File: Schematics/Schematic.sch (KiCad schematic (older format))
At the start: 14 parts

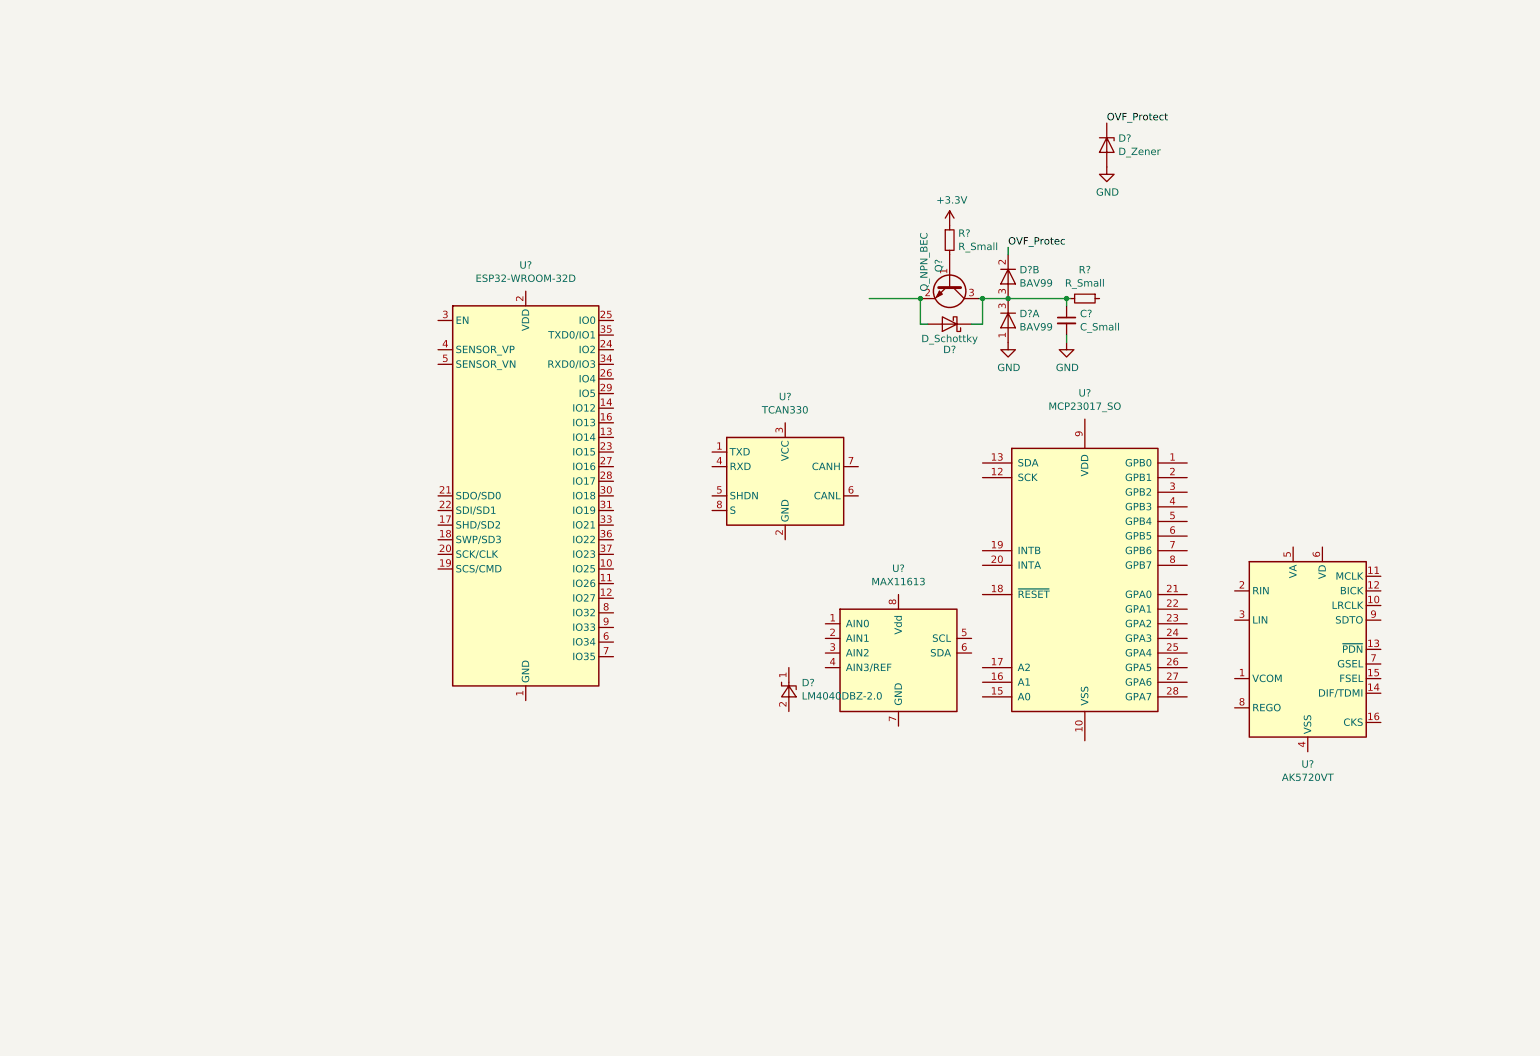
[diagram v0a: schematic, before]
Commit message: Whheee, parts!
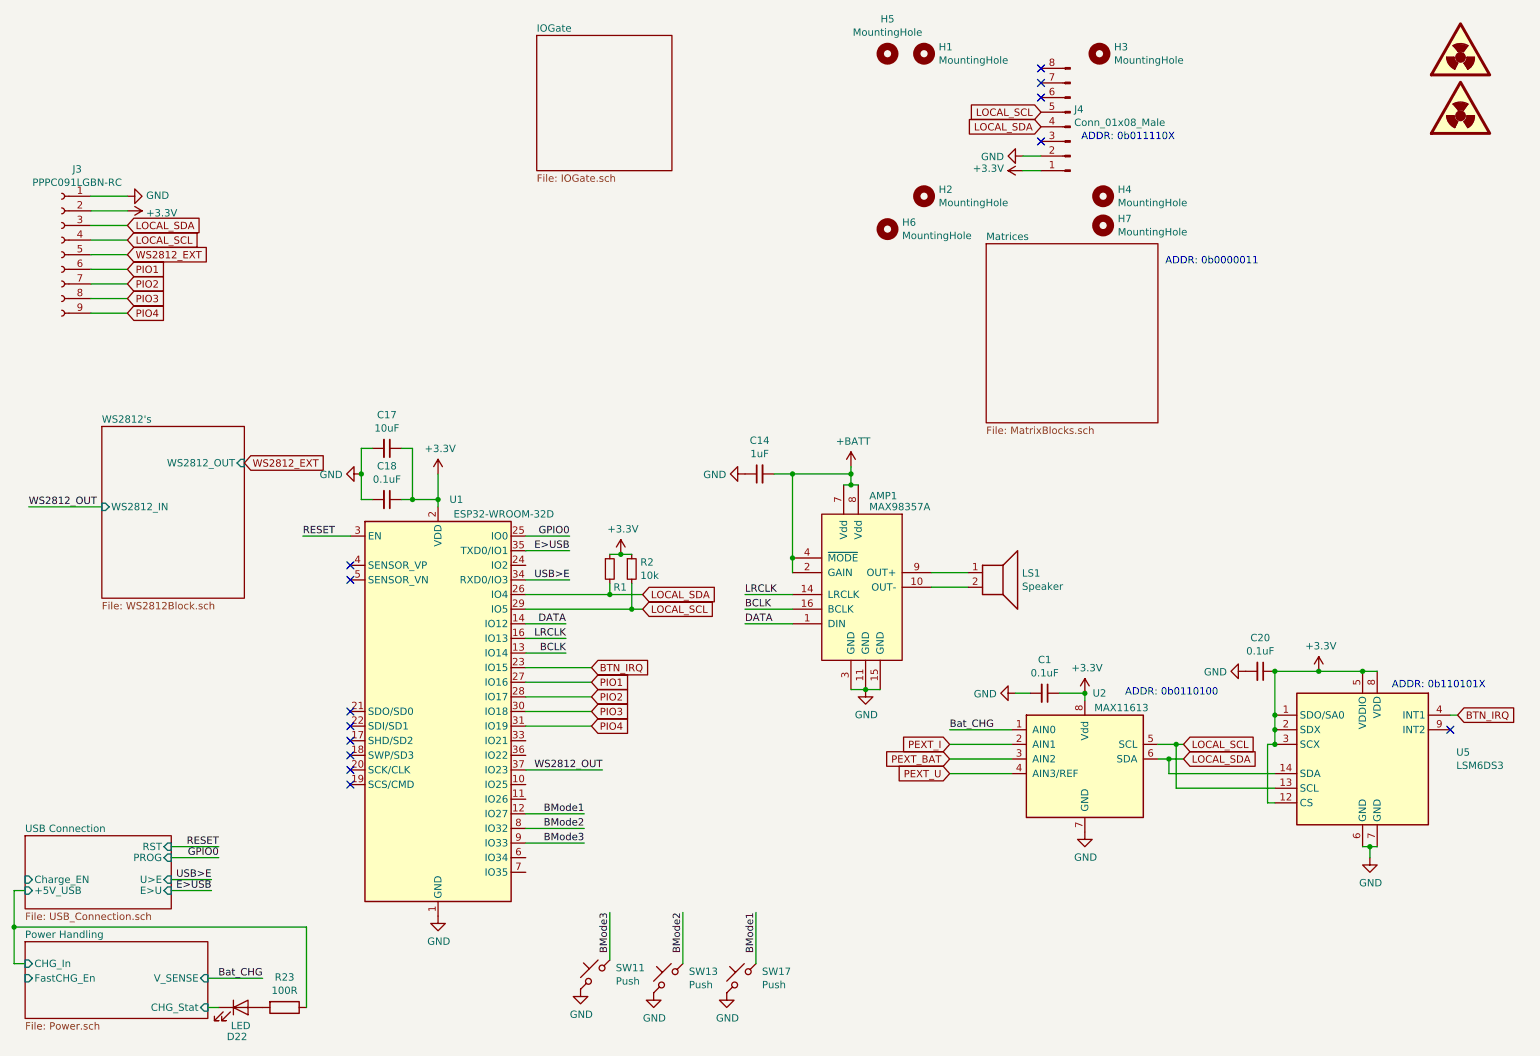
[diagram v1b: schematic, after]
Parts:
- removed C?: C_Small, Capacitor_SMD:C_0805_2012Metric, symbol Device:C_Small
- removed D? (x2): BAV99, Package_TO_SOT_SMD:SOT-23, symbol Diode:BAV99
- removed D?: D_Zener, symbol Device:D_Zener
- removed D?: D_Schottky, symbol Device:D_Schottky
- removed D?: LM4040DBZ-2.0, Package_TO_SOT_SMD:SOT-23, symbol Reference_Voltage:LM4040DBZ-2.0
- removed Q?: Q_NPN_BEC, Package_TO_SOT_SMD:SOT-23, symbol Device:Q_NPN_BEC
- removed R?: R_Small, Resistor_SMD:R_0805_2012Metric, symbol Device:R_Small
- removed R?: R_Small, symbol Device:R_Small
- removed U?: MAX11613, Package_SO:MSOP-8_3x3mm_P0.65mm, symbol Analog_ADC:MAX11613
- removed U?: MCP23017_SO, Package_SO:SOIC-28W_7.5x17.9mm_P1.27mm, symbol Interface_Expansion:MCP23017_SO
- removed U?: TCAN330, symbol Interface_CAN_LIN:TCAN330
- removed U?: AK5720VT, Package_SO:TSSOP-16_4.4x5mm_P0.65mm, symbol Audio:AK5720VT
- added AMP1: MAX98357A, Package_DFN_QFN:QFN-16-1EP_3x3mm_P0.5mm_EP2.7x2.7mm_ThermalVias, symbol XasParts:MAX98357A
- added C1, C18, C20: 0.1uF, Capacitor_SMD:C_0805_2012Metric, symbol Device:C_Small
- added C14: 1uF, Capacitor_SMD:C_0805_2012Metric, symbol Device:C_Small
- added C17: 10uF, Capacitor_SMD:C_0805_2012Metric, symbol Device:C_Small
- added D22: LED, LED_SMD:LED_0805_2012Metric, symbol Device:LED
- added H1, H2, H3, H4, H5, H6, H7: MountingHole, MountingHole:MountingHole_3.2mm_M3, symbol Mechanical:MountingHole
- added J3: PPPC091LGBN-RC, Connector_PinSocket_2.54mm:PinSocket_1x09_P2.54mm_Horizontal, symbol Connector:Conn_01x09_Female
- added J4: Conn_01x08_Male, Connector_PinHeader_2.54mm:PinHeader_1x08_P2.54mm_Vertical, symbol Connector:Conn_01x08_Male
- added LS1: Speaker, Connector_PinHeader_2.00mm:PinHeader_1x02_P2.00mm_Vertical, symbol Device:Speaker
- added R1: R_Small, Resistor_SMD:R_0805_2012Metric, symbol Device:R_Small
- added R2: 10k, Resistor_SMD:R_0805_2012Metric, symbol Device:R_Small
- added R23: 100R, Resistor_SMD:R_0805_2012Metric, symbol Device:R
- added SW11, SW13, SW17: Push, Button_Switch_SMD:SW_SPST_PTS645, symbol Switch:SW_Push_45deg
- added SYM1: SYM_Radioactive_Large, XasParts:Xas_Logo, symbol Graphic:SYM_Radioactive_Large
- added SYM2: SYM_Radioactive_Large, XasParts:Hackaday_Link, symbol Graphic:SYM_Radioactive_Large
- added U2: MAX11613, Package_SO:MSOP-8_3x3mm_P0.65mm, symbol Analog_ADC:MAX11613
- added U5: LSM6DS3, Package_LGA:LGA-14_3x2.5mm_P0.5mm_LayoutBorder3x4y, symbol Sensor_Motion:LSM6DS3
- U1: renamed from U?; footprint RF_Module:ESP32-WROOM-32 -> RF_Module:ESP32-WROOM-32U
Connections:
- net labels added: +BATT, BCLK, BMode1, BMode2, BMode3, BTN_IRQ, Bat_CHG, DATA, E>USB, GPIO0, LOCAL_SCL, LOCAL_SDA, LRCLK, PEXT_BAT, PEXT_I, PEXT_U, PIO1, PIO2, PIO3, PIO4, RESET, USB>E, WS2812_EXT, WS2812_OUT
- net labels removed: OVF_Protec, OVF_Protect
- wire segments 12 -> 104
- no-connect marks 0 -> 13
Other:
- note added: "ADDR: 0b0000011"
- note added: "ADDR: 0b0110100"
- note added: "ADDR: 0b011110X"
- note added: "ADDR: 0b110101X\n"
- moved on the sheet: U1
